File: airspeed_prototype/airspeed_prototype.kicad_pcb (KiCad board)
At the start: 2 copper layers, 29.2 x 34.3 mm, 4 parts, among them J1 Conn_01x03_Pin, J2 Conn_01x10_Pin

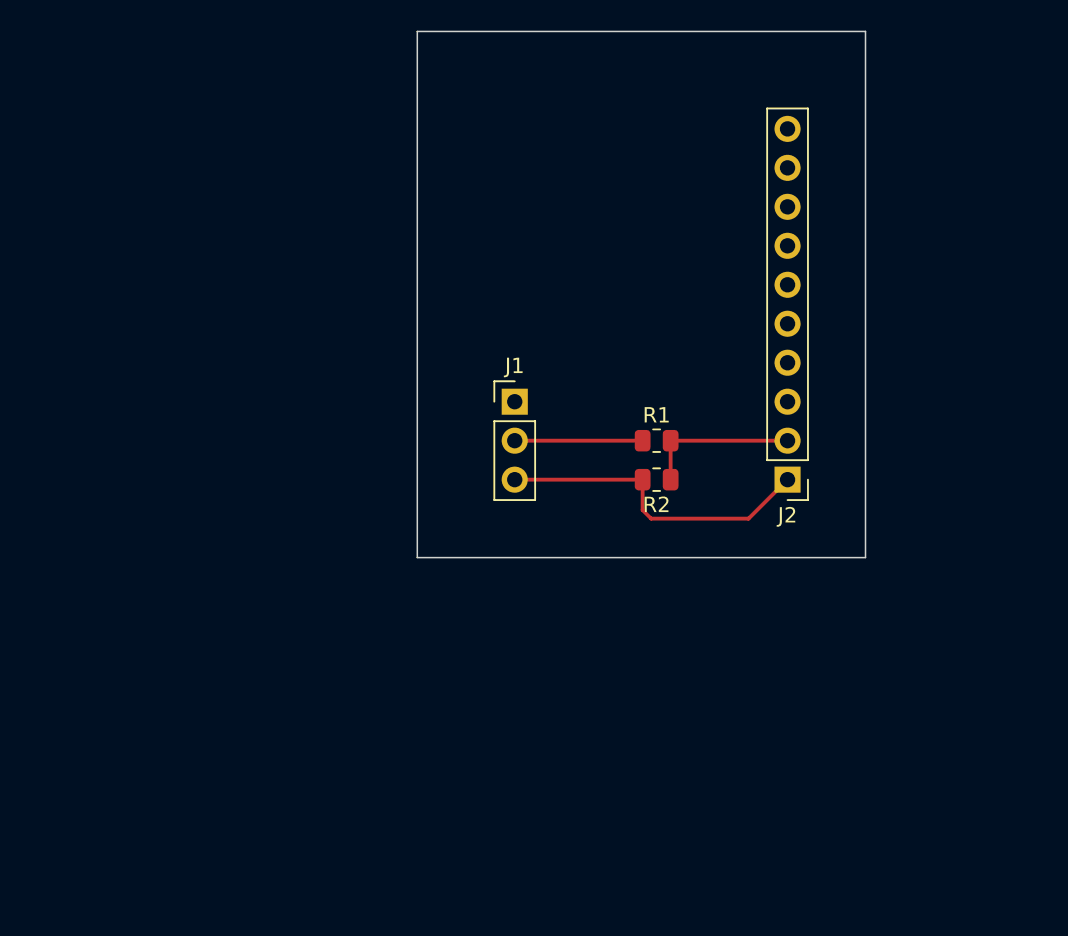
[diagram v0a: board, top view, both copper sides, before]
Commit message: update the schematic and pcb
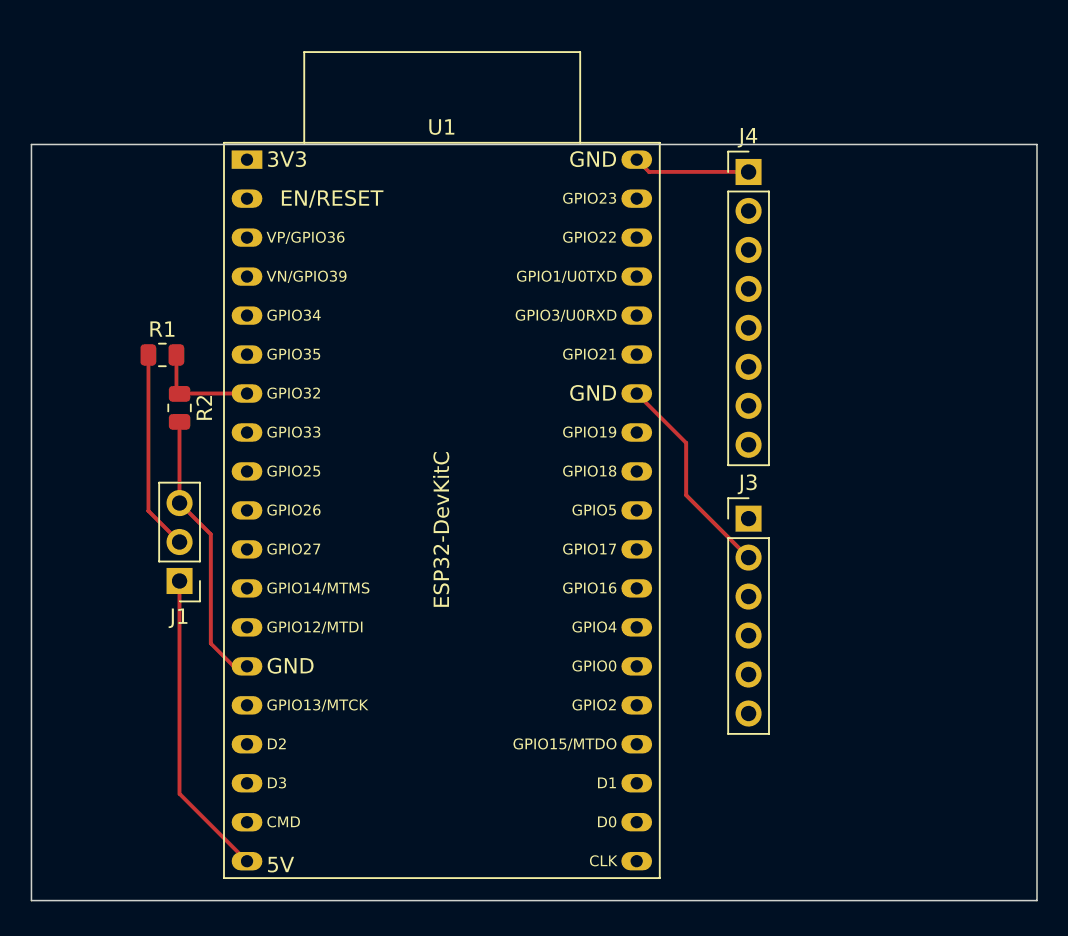
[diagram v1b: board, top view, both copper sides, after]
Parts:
- removed J2: Conn_01x10_Pin, Connector_PinHeader_2.54mm:PinHeader_1x10_P2.54mm_Vertical
- added J3: Conn_01x06_Pin, Connector_PinHeader_2.54mm:PinHeader_1x06_P2.54mm_Vertical, F.Cu at (121.9, 68.6)
- added J4: Conn_01x08_Pin, Connector_PinHeader_2.54mm:PinHeader_1x08_P2.54mm_Vertical, F.Cu at (121.9, 46.0)
- added U1: ESP32-DevKitC, PCM_Espressif:ESP32-DevKitC, F.Cu at (89.2, 45.2)
- moved R1 32.7 mm to (83.7, 57.9)
- moved R2 31.4 mm to (84.8, 61.4), turned to -90 degrees
- moved J1 24.8 mm to (84.8, 72.6), turned to 180 degrees
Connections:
- J1 pad 1: +5V -> /5V
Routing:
- net /5V: track 0.00 -> 20.1 mm
- net GND: track 21.0 -> 39.6 mm
- net Net-(J1-Pin_2): track 8.33 -> 13.0 mm
- net Net-(U1-32K_XP/GPIO32/ADC1_CH4): track 10.2 -> 7.03 mm
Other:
- board size 29.2 x 34.3 mm -> 65.5 x 49.3 mm

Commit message: updates
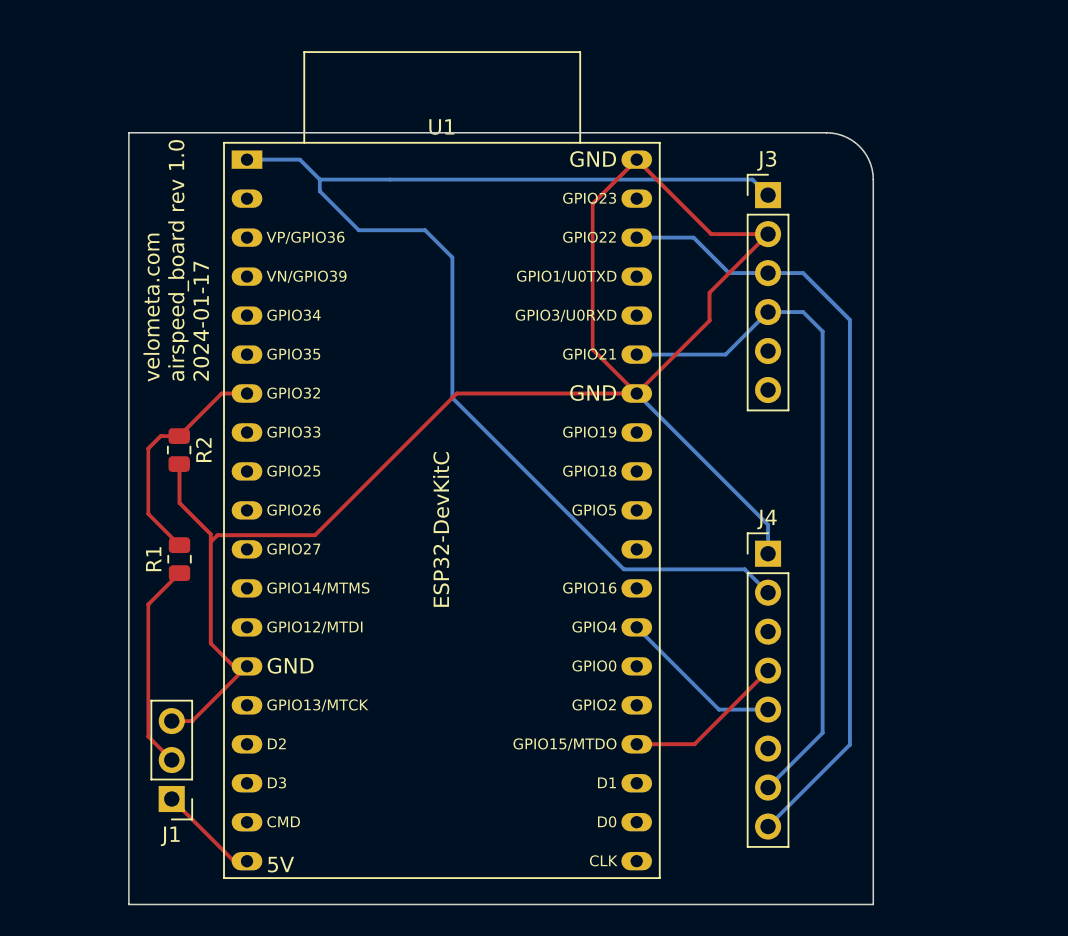
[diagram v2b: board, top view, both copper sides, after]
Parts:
- moved J4 24.9 mm to (123.2, 70.9)
- moved J3 21.1 mm to (123.2, 47.5)
- moved J1 14.2 mm to (84.3, 86.9)
- moved R1 13.4 mm to (84.8, 71.2), turned to 90 degrees
- moved R2 2.75 mm to (84.8, 64.1)
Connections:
- net /5V renamed +5V
- J3 pad 1: unconnected-(J3-VCC-Pad1) -> +3.3V
- J3 pad 3: unconnected-(J3-SCL-Pad3) -> Net-(J3-SCL)
- J3 pad 4: unconnected-(J3-SDA-Pad4) -> Net-(J3-SDA)
- J4 pad 2: unconnected-(J4-VCC-Pad2) -> +3.3V
- J4 pad 4: unconnected-(J4-INT1-Pad4) -> Net-(J4-INT1)
- J4 pad 5: unconnected-(J4-INT2-Pad5) -> Net-(J4-INT2)
- J4 pad 7: unconnected-(J4-SDA-Pad7) -> Net-(J3-SDA)
- J4 pad 8: unconnected-(J4-SCL-Pad8) -> Net-(J3-SCL)
- U1 pad 1: /3.3V -> +3.3V
- U1 pad 23: unconnected-(U1-MTDO/GPIO15/ADC2_CH3-Pad23) -> Net-(J4-INT1)
- U1 pad 26: unconnected-(U1-ADC2_CH0/GPIO4-Pad26) -> Net-(J4-INT2)
- U1 pad 33: unconnected-(U1-GPIO21-Pad33) -> Net-(J3-SDA)
- U1 pad 36: unconnected-(U1-GPIO22-Pad36) -> Net-(J3-SCL)
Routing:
- net +3.3V: track 0.00 -> 81.1 mm
- net GND: track 39.6 -> 109.8 mm
- net Net-(J3-SCL): track 0.00 -> 51.3 mm
- net Net-(J3-SDA): track 0.00 -> 45.8 mm
- net +5V: track 20.1 -> 6.58 mm
- net Net-(J4-INT2): track 0.00 -> 10.8 mm
- net Net-(J4-INT1): track 0.00 -> 10.5 mm
- net Net-(U1-32K_XP/GPIO32/ADC1_CH4): track 7.03 -> 15.1 mm
- net Net-(J1-Pin_2): track 13.0 -> 13.6 mm
- net unconnected-(J4-CS-Pad3): track 0.00 -> 0.51 mm
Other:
- board size 65.5 x 49.3 mm -> 48.5 x 50.3 mm
- board text added: "velometa.com airspeed_board rev 1.0 2024-01-17"

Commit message: updates to pcb
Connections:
- net Net-(J3-SCL) renamed SCL
- net Net-(J3-SDA) renamed SDA
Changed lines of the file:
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@@
   (net 1 "Net-(J1-Pin_2)")
   (net 2 "GND")
-  (net 3 "Net-(J3-SCL)")
-  (net 4 "Net-(J3-SDA)")
+  (net 3 "SCL")
+  (net 4 "SDA")
   (net 5 "Net-(J4-INT1)")
   (net 6 "Net-(J4-INT2)")
@@
       (net 13 "unconnected-(J4-SDO-Pad6)") (pinfunction "SDO") (pintype "passive+no_connect"))
     (pad "7" thru_hole oval (at 0 15.24) (size 1.7 1.7) (drill 1) (layers "*.Cu" "*.Mask")
-      (net 4 "Net-(J3-SDA)") (pinfunction "SDA") (pintype "passive"))
+      (net 4 "SDA") (pinfunction "SDA") (pintype "passive"))
     (pad "8" thru_hole oval (at 0 17.78) (size 1.7 1.7) (drill 1) (layers "*.Cu" "*.Mask")
-      (net 3 "Net-(J3-SCL)") (pinfunction "SCL") (pintype "passive"))
+      (net 3 "SCL") (pinfunction "SCL") (pintype "passive"))
     (model "${KICAD6_3DMODEL_DIR}/Connector_PinHeader_2.54mm.3dshapes/PinHeader_1x08_P2.54mm_Vertical.wrl"
       (offset (xyz 0 0 0))
@@
       (net 2 "GND") (pinfunction "GND") (pintype "passive"))
     (pad "33" thru_hole oval (at 25.4 12.7 270) (size 1.2 2) (drill 0.8) (layers "*.Cu" "*.Mask")
-      (net 4 "Net-(J3-SDA)") (pinfunction "SDA") (pintype "bidirectional"))
+      (net 4 "SDA") (pinfunction "SDA") (pintype "bidirectional"))
     (pad "34" thru_hole oval (at 25.4 10.16 270) (size 1.2 2) (drill 0.8) (layers "*.Cu" "*.Mask")
       (net 39 "unconnected-(U1-U0RXD{slash}GPIO3-Pad34)") (pinfunction "U0RXD/GPIO3") (pintype "bidirectional+no_connect"))
@@
       (net 40 "unconnected-(U1-U0TXD{slash}GPIO1-Pad35)") (pinfunction "U0TXD/GPIO1") (pintype "bidirectional+no_connect"))
     (pad "36" thru_hole oval (at 25.4 5.08 270) (size 1.2 2) (drill 0.8) (layers "*.Cu" "*.Mask")
-      (net 3 "Net-(J3-SCL)") (pinfunction "SCL") (pintype "bidirectional"))
+      (net 3 "SCL") (pinfunction "SCL") (pintype "bidirectional"))
     (pad "37" thru_hole oval (at 25.4 2.54 270) (size 1.2 2) (drill 0.8) (layers "*.Cu" "*.Mask")
       (net 41 "unconnected-(U1-GPIO23-Pad37)") (pinfunction "GPIO23") (pintype "bidirectional+no_connect"))
@@
       (net 2 "GND") (pinfunction "GND") (pintype "passive"))
     (pad "3" thru_hole oval (at 0 5.08) (size 1.7 1.7) (drill 1) (layers "*.Cu" "*.Mask")
-      (net 3 "Net-(J3-SCL)") (pinfunction "SCL") (pintype "passive"))
+      (net 3 "SCL") (pinfunction "SCL") (pintype "passive"))
     (pad "4" thru_hole oval (at 0 7.62) (size 1.7 1.7) (drill 1) (layers "*.Cu" "*.Mask")
-      (net 4 "Net-(J3-SDA)") (pinfunction "SDA") (pintype "passive"))
+      (net 4 "SDA") (pinfunction "SDA") (pintype "passive"))
     (pad "5" thru_hole oval (at 0 10.16) (size 1.7 1.7) (drill 1) (layers "*.Cu" "*.Mask")
       (net 10 "unconnected-(J3-CSB-Pad5)") (pinfunction "CSB") (pintype "passive+no_connect"))
